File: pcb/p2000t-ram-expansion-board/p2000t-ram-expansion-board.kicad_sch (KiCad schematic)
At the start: 23 parts, among them J1 EXPANSION BOARD, J2 POWER, J3 TERMINAL, U1 74HC04, U2 CY62256-70PC, U3 74HC00, U4 CY62256-70PC, U5 74HC688, U6 74HC32, U7 74HC173, U8 74HC245, U9 74HC157

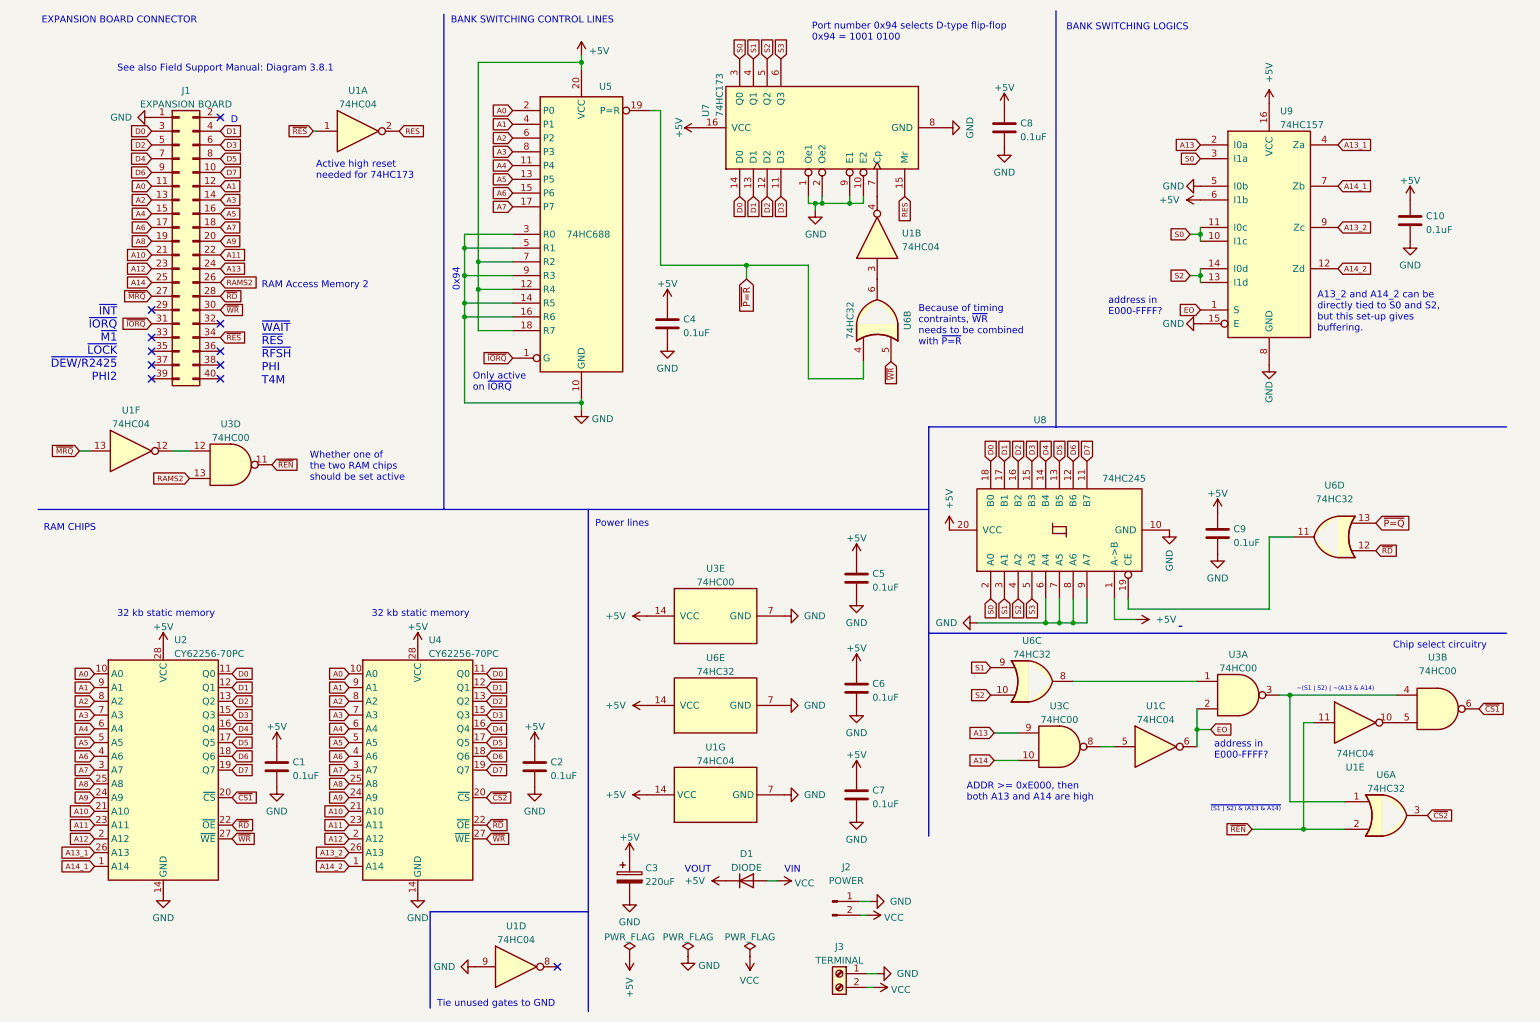
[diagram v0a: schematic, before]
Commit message: Revising PCBs
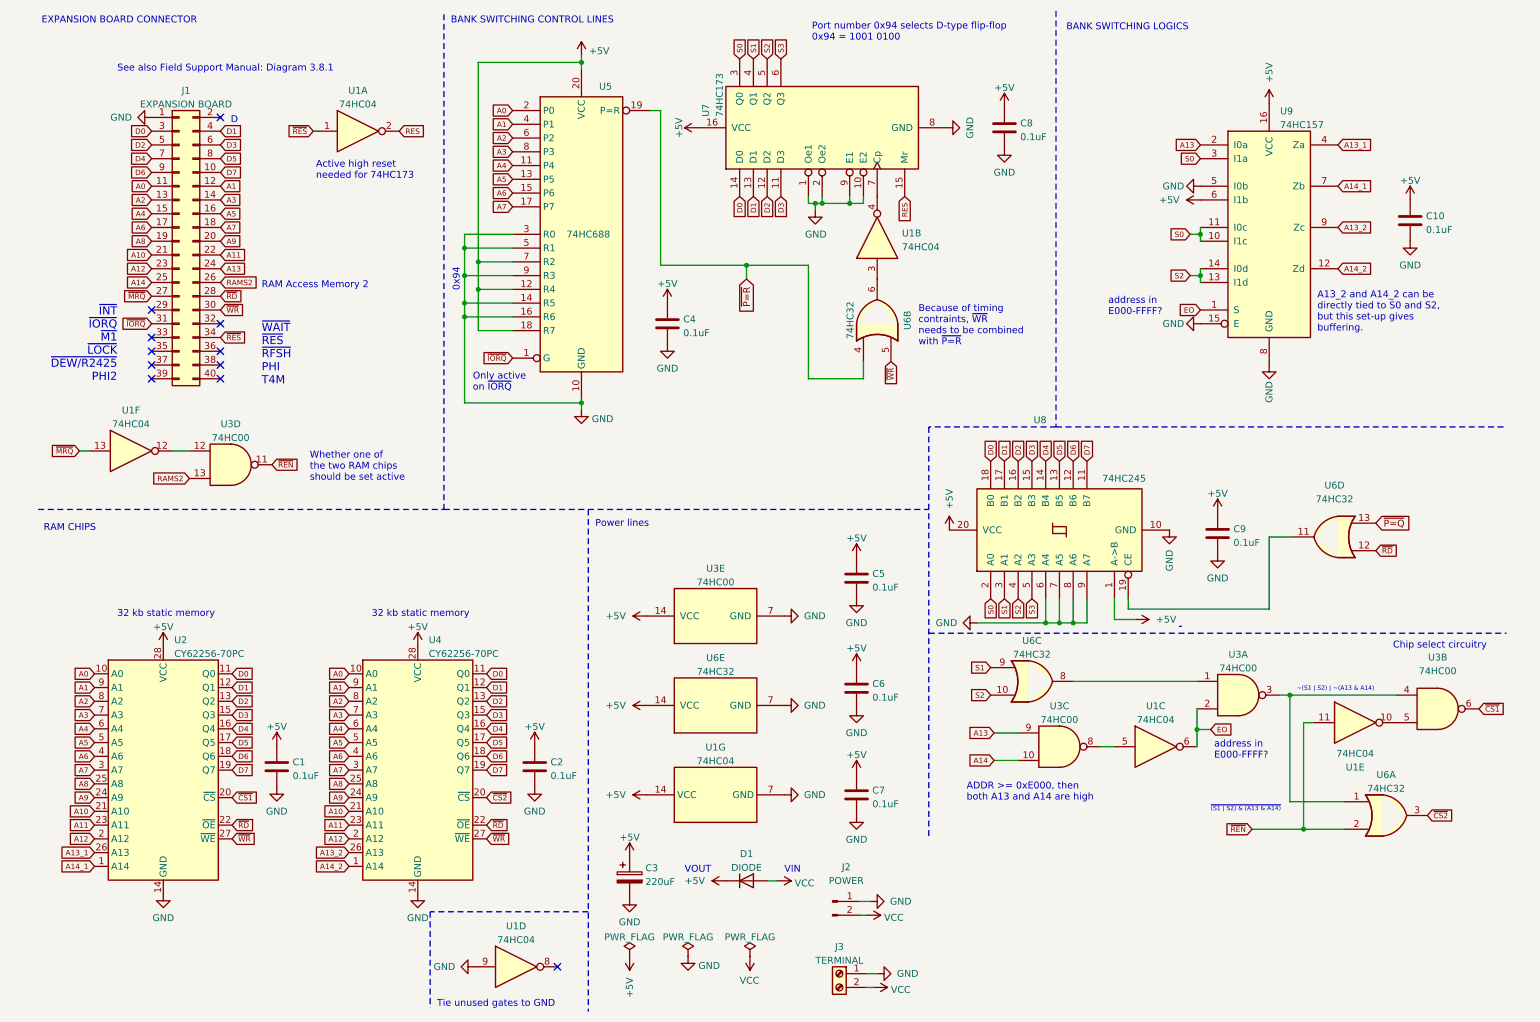
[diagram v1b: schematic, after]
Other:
- title: P2000T RAM expansion board -> Philips P2000T 64kb memory expansion board
